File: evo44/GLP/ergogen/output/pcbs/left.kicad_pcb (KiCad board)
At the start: 2 copper layers, 138.8 x 113.9 mm, 68 parts

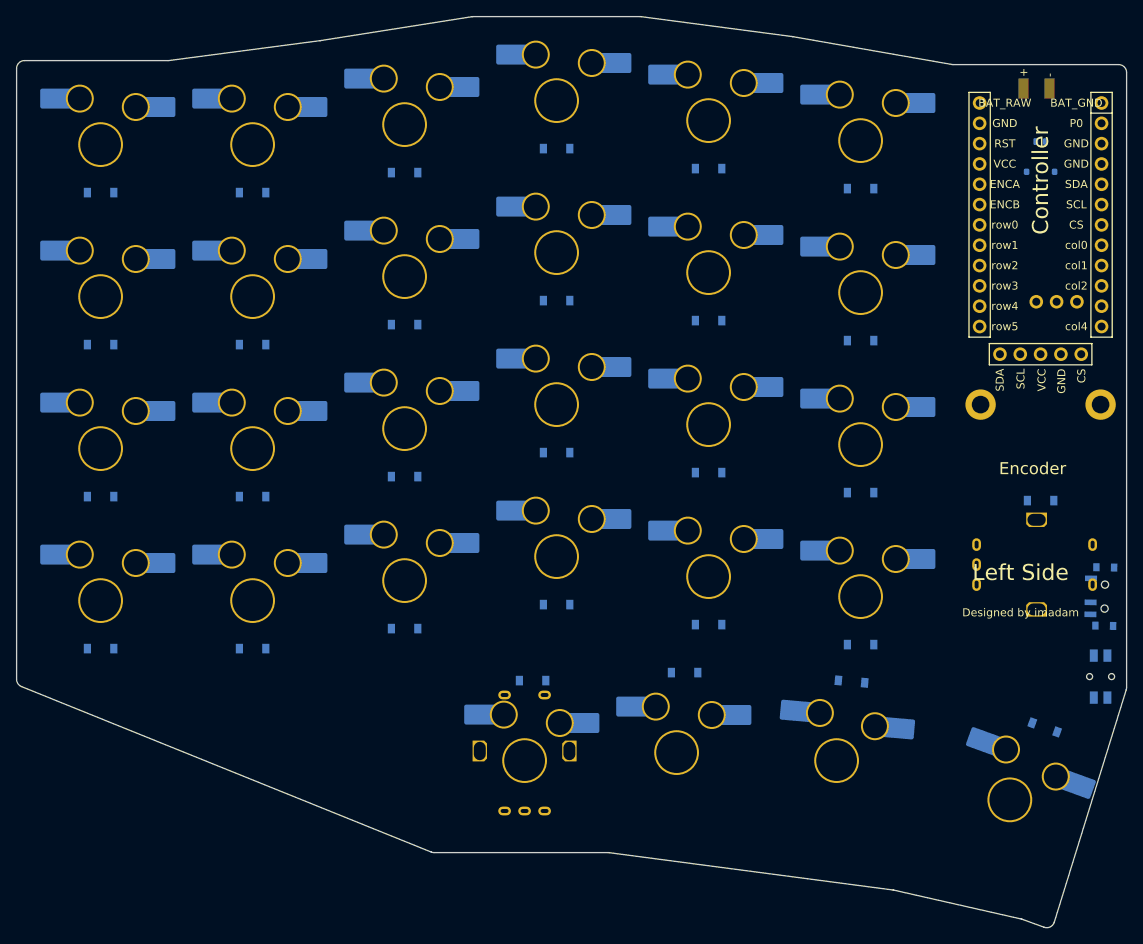
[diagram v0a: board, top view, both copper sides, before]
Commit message: ok
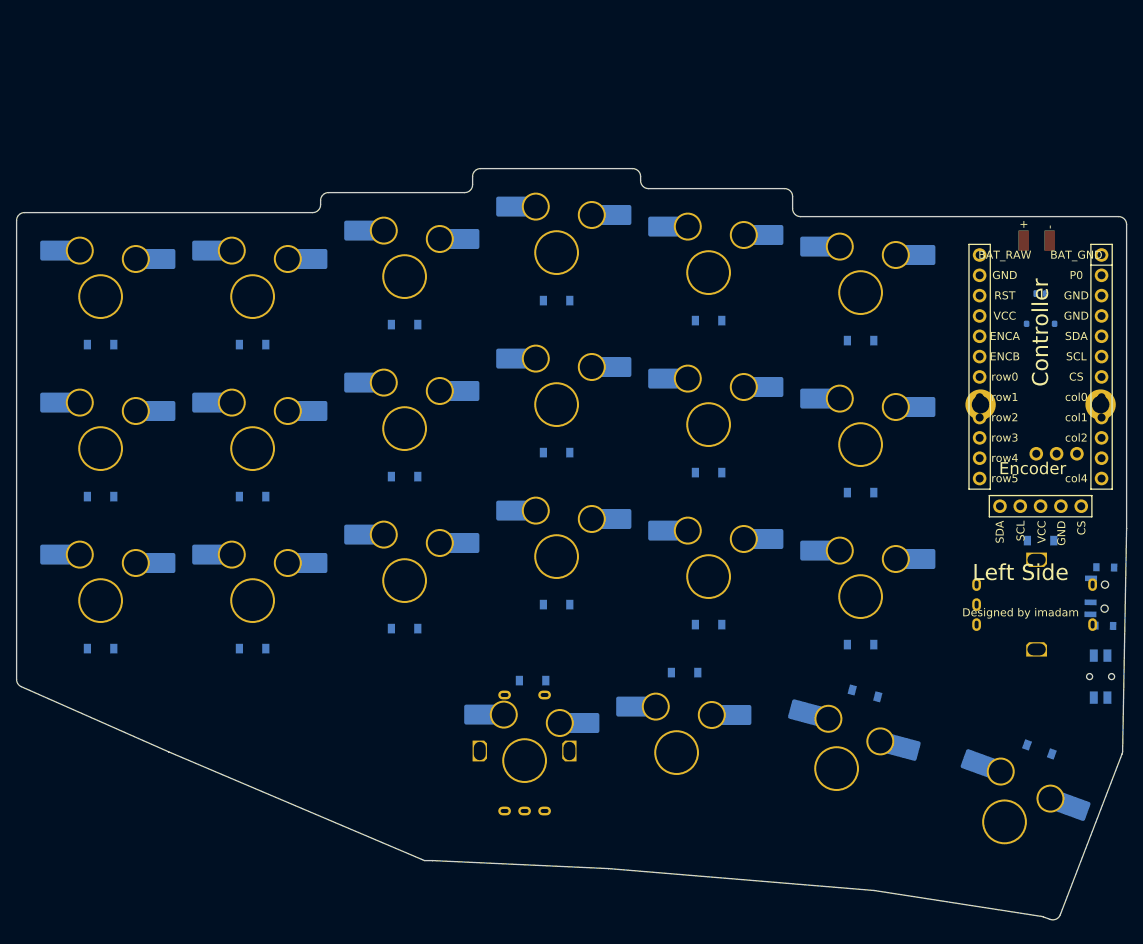
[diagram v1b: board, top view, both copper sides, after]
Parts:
- removed D24, D25, D26, D27, D28, D29: , ceoloide:diode_tht_sod123
- removed S23, S24, S25, S26, S27, S28: , ceoloide:switch_gateron_ks27_ks33
- moved S20 79.1 mm to (122.0, 150.0)
- moved D16 72.7 mm to (145.0, 136.5)
- moved S16 72.7 mm to (145.0, 130.5)
- moved S19 65.2 mm to (103.0, 151.0)
- moved D20 63.1 mm to (123.0, 140.0)
- moved D4 60.1 mm to (69.0, 137.0)
- moved S4 60.1 mm to (69.0, 131.0)
- moved S22 50.5 mm to (163.0, 158.7), turned to 160 degrees
- moved D19 50.1 mm to (104.0, 141.0)
- moved D7 40.3 mm to (88.0, 134.5)
- moved D8 40.3 mm to (88.0, 115.5)
- moved S7 40.3 mm to (88.0, 128.5)
- moved S8 40.3 mm to (88.0, 109.5)
- moved D22 39.1 mm to (167.4, 149.6), turned to -20 degrees
- moved D9 38.0 mm to (88.0, 96.5)
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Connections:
- D10 pad 1: row2 -> row3
- D10 pad 2: ring_home -> middle_bottom
- D11 pad 1: row1 -> row2
- D11 pad 2: ring_top -> middle_home
- D12 pad 1: row0 -> row1
- D12 pad 2: ring_num -> middle_top
- D13 pad 2: middle_bottom -> index_bottom
- D14 pad 2: middle_home -> index_home
- D15 pad 2: middle_top -> index_top
- D16 pad 1: row0 -> row3
- D16 pad 2: middle_num -> inner_bottom
- D17 pad 1: row3 -> row2
- D17 pad 2: index_bottom -> inner_home
- D18 pad 1: row2 -> row1
- D18 pad 2: index_home -> inner_top
- D19 pad 1: row1 -> row4
- D19 pad 2: index_top -> inner_cluster
- D20 pad 1: row0 -> row4
- D20 pad 2: index_num -> home_cluster
- D21 pad 1: row3 -> row4
- D21 pad 2: inner_bottom -> layer_cluster
- D22 pad 1: row2 -> row4
- D22 pad 2: inner_home -> space_cluster
- D23 pad 1: row1 -> row2
- D23 pad 2: inner_top -> scrollwheel_enc
- D4 pad 1: row0 -> row3
- D4 pad 2: outer_num -> pinky_bottom
- D5 pad 1: row3 -> row2
- D5 pad 2: pinky_bottom -> pinky_home
- D6 pad 1: row2 -> row1
- D6 pad 2: pinky_home -> pinky_top
- D7 pad 1: row1 -> row3
- D7 pad 2: pinky_top -> ring_bottom
- D8 pad 1: row0 -> row2
- D8 pad 2: pinky_num -> ring_home
- D9 pad 1: row3 -> row1
- D9 pad 2: ring_bottom -> ring_top
- S10 pad 1: col2 -> col3
- S10 pad 2: ring_home -> middle_bottom
- S11 pad 1: col2 -> col3
- S11 pad 2: ring_top -> middle_home
- S12 pad 1: col2 -> col3
- S12 pad 2: ring_num -> middle_top
- S13 pad 1: col3 -> col4
- S13 pad 2: middle_bottom -> index_bottom
- S14 pad 1: col3 -> col4
- S14 pad 2: middle_home -> index_home
- S15 pad 1: col3 -> col4
- S15 pad 2: middle_top -> index_top
- S16 pad 1: col3 -> col5
- S16 pad 2: middle_num -> inner_bottom
- S17 pad 1: col4 -> col5
- S17 pad 2: index_bottom -> inner_home
- S18 pad 1: col4 -> col5
- S18 pad 2: index_home -> inner_top
- S19 pad 1: col4 -> col2
- S19 pad 2: index_top -> inner_cluster
- S20 pad 1: col4 -> col3
- S20 pad 2: index_num -> home_cluster
- S21 pad 1: col5 -> col4
- S21 pad 2: inner_bottom -> layer_cluster
- S22 pad 2: inner_home -> space_cluster
- S4 pad 1: col0 -> col1
- S4 pad 2: outer_num -> pinky_bottom
- S5 pad 2: pinky_bottom -> pinky_home
- S6 pad 2: pinky_home -> pinky_top
- S7 pad 1: col1 -> col2
- S7 pad 2: pinky_top -> ring_bottom
- S8 pad 1: col1 -> col2
- S8 pad 2: pinky_num -> ring_home
- S9 pad 2: ring_bottom -> ring_top
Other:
- board size 138.8 x 113.9 mm -> 138.8 x 93.9 mm
